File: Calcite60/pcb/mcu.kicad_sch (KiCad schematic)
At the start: 13 parts, among them SW2 RESET, U4 E73-2G4M08S1C, Y1 32.768kHz

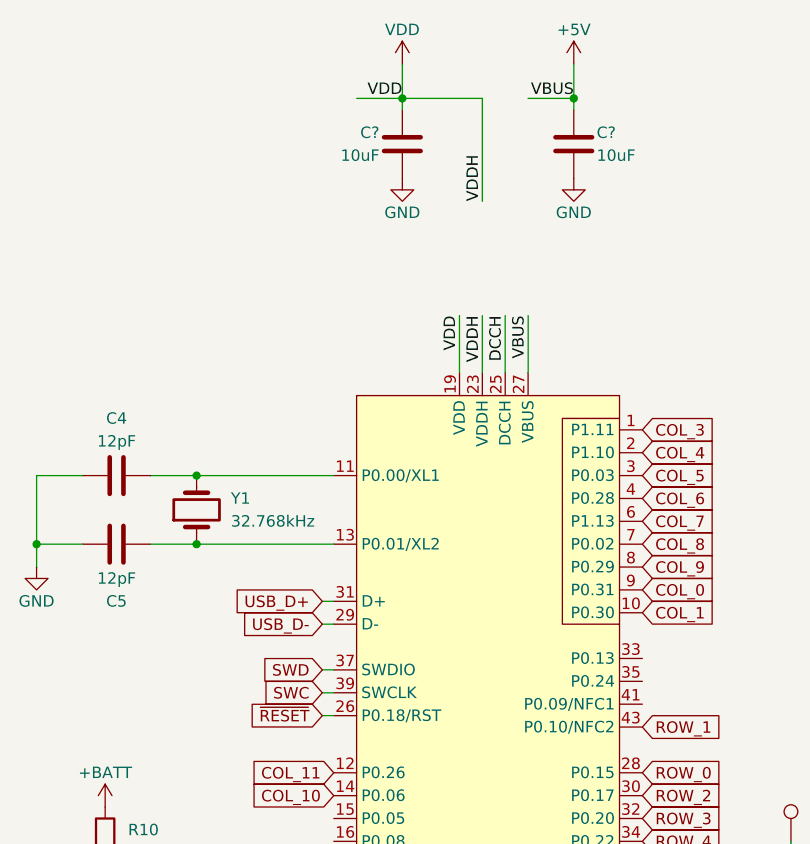
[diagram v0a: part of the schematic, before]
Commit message: Update BOM
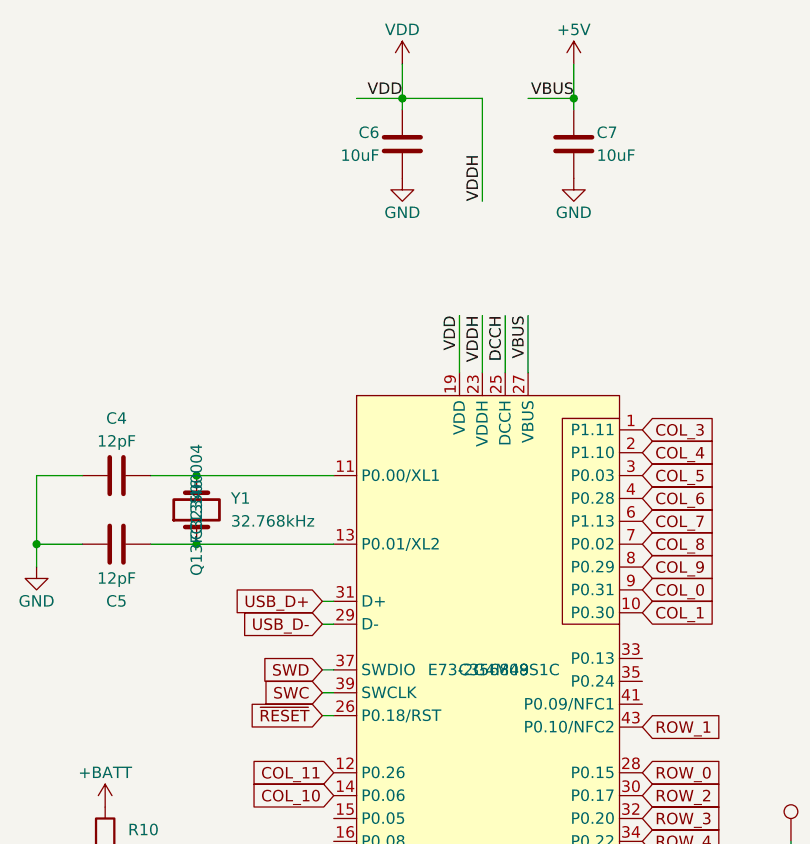
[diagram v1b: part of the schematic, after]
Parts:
- C4, C5: LCSC (none) -> C38523; MFR. Part # (none) -> CL10C120JB8NNNC
- C6, C7: renamed from C?; LCSC (none) -> C19702; MFR. Part # (none) -> CL10A106KP8NNNC
- R10: LCSC C11702 -> C23252; MFR. Part # 0402WGF1001TCE -> 0603WAF8203T5E
- R7: LCSC C25744 -> C25804; MFR. Part # 0402WGF1002TCE -> 0603WAF1002T5E
- R9: LCSC C11702 -> C22976; MFR. Part # 0402WGF1001TCE -> 0603WAF2004T5E
- U4: LCSC (none) -> C356849; MFR. Part # (none) -> E73-2G4M08S1C
- Y1: LCSC (none) -> C32346; MFR. Part # (none) -> Q13FC13500004
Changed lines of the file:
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@@
 (kicad_sch
-	(version 20231120)
+	(version 20250114)
 	(generator "eeschema")
-	(generator_version "8.0")
+	(generator_version "9.0")
 	(paper "A4")
 	(junction
@@
 	(label "VDD"
 		(at 163.83 71.12 270)
-		(fields_autoplaced yes)
 		(effects
 			(font
@@
 	(label "VDDH"
 		(at 166.37 71.12 270)
-		(fields_autoplaced yes)
 		(effects
 			(font
@@
 	(label "VDD"
 		(at 157.48 46.99 180)
-		(fields_autoplaced yes)
 		(effects
 			(font
@@
 	(label "VBUS"
 		(at 176.53 46.99 180)
-		(fields_autoplaced yes)
 		(effects
 			(font
@@
 	(label "Battery_sense"
 		(at 124.46 134.62 0)
-		(fields_autoplaced yes)
 		(effects
 			(font
@@
 	(label "VDDH"
 		(at 166.37 58.42 90)
-		(fields_autoplaced yes)
 		(effects
 			(font
@@
 	(label "DCCH"
 		(at 168.91 71.12 270)
-		(fields_autoplaced yes)
 		(effects
 			(font
@@
 	(label "VBUS"
 		(at 171.45 71.12 270)
-		(fields_autoplaced yes)
 		(effects
 			(font
@@
 			)
 		)
-		(property "MFR. Part #" ""
+		(property "MFR. Part #" "CL10C120JB8NNNC"
 			(at 125.73 96.52 0)
 			(effects
@@
 			)
 		)
-		(property "LCSC" ""
+		(property "LCSC" "C38523"
 			(at 125.73 96.52 0)
 			(effects
@@
 			)
 		)
+		(property "LCSC" "C356849"
+			(at 167.64 110.49 0)
+			(effects
+				(font
+					(size 1.27 1.27)
+				)
+			)
+		)
+		(property "MFR. Part #" "E73-2G4M08S1C"
+			(at 167.64 110.49 0)
+			(effects
+				(font
+					(size 1.27 1.27)
+				)
+			)
+		)
 		(pin "1"
 		)
@@
 		(on_board yes)
 		(dnp no)
-		(property "Reference" "C?"
+		(property "Reference" "C7"
 			(at 179.07 50.8 0)
 			(effects
@@
 			)
 		)
-		(property "MFR. Part #" ""
+		(property "MFR. Part #" "CL10A106KP8NNNC"
 			(at 176.53 52.07 0)
 			(effects
@@
 			)
 		)
-		(property "LCSC" ""
+		(property "LCSC" "C19702"
 			(at 176.53 52.07 0)
 			(effects
@@
 		(on_board yes)
 		(dnp no)
-		(property "Reference" "C?"
+		(property "Reference" "C6"
 			(at 154.94 50.8 0)
 			(effects
@@
 			)
 		)
-		(property "MFR. Part #" ""
+		(property "MFR. Part #" "CL10A106KP8NNNC"
 			(at 157.48 52.07 0)
 			(effects
@@
 			)
 		)
-		(property "LCSC" ""
+		(property "LCSC" "C19702"
 			(at 157.48 52.07 0)
 			(effects
@@
 			)
 		)
-		(property "MFR. Part #" "0402WGF1001TCE "
+		(property "MFR. Part #" "0603WAF8203T5E"
 			(at 124.46 129.54 0)
 			(effects
@@
 			)
 		)
-		(property "LCSC" "C11702"
+		(property "LCSC" "C23252"
 			(at 124.46 129.54 0)
 			(effects
@@
 				)
 				(hide yes)
+			)
+		)
+		(property "LCSC" "C32346"
+			(at 134.62 92.71 0)
+			(effects
+				(font
+					(size 1.27 1.27)
+				)
+			)
+		)
+		(property "MFR. Part #" "Q13FC13500004"
+			(at 134.62 92.71 0)
+			(effects
+				(font
+					(size 1.27 1.27)
+				)
 			)
 		)
@@
 			)
 		)
-		(property "MFR. Part #" "0402WGF1002TCE "
+		(property "MFR. Part #" "0603WAF1002T5E"
 			(at 82.55 76.2 0)
 			(effects
@@
 			)
 		)
-		(property "LCSC" "C25744"
+		(property "LCSC" "C25804"
 			(at 82.55 76.2 0)
 			(effects
@@
 			)
 		)
-		(property "MFR. Part #" ""
+		(property "MFR. Part #" "CL10C120JB8NNNC"
 			(at 125.73 88.9 0)
 			(effects
@@
 			)
 		)
-		(property "LCSC" ""
+		(property "LCSC" "C38523"
 			(at 125.73 88.9 0)
 			(effects
@@
 			)
 		)
-		(property "MFR. Part #" "0402WGF1001TCE "
+		(property "MFR. Part #" "0603WAF2004T5E"
 			(at 124.46 139.7 0)
 			(effects
@@
 			)
 		)
-		(property "LCSC" "C11702"
+		(property "LCSC" "C22976"
 			(at 124.46 139.7 0)
 			(effects
